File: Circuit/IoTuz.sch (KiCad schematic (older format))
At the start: 29 parts, among them P1 Alligator Connector, P2 BATTERY, P3 USB_5PIN_SHELL, P4 LED_1, P5 LED_2, P6 CONN_01X20, P7 CONN_01X20, Q1 S8050, Q2 S8050, Q3 FDN340P, SW5 RESET, U1 CP2102, U2 ESP32-WROOM

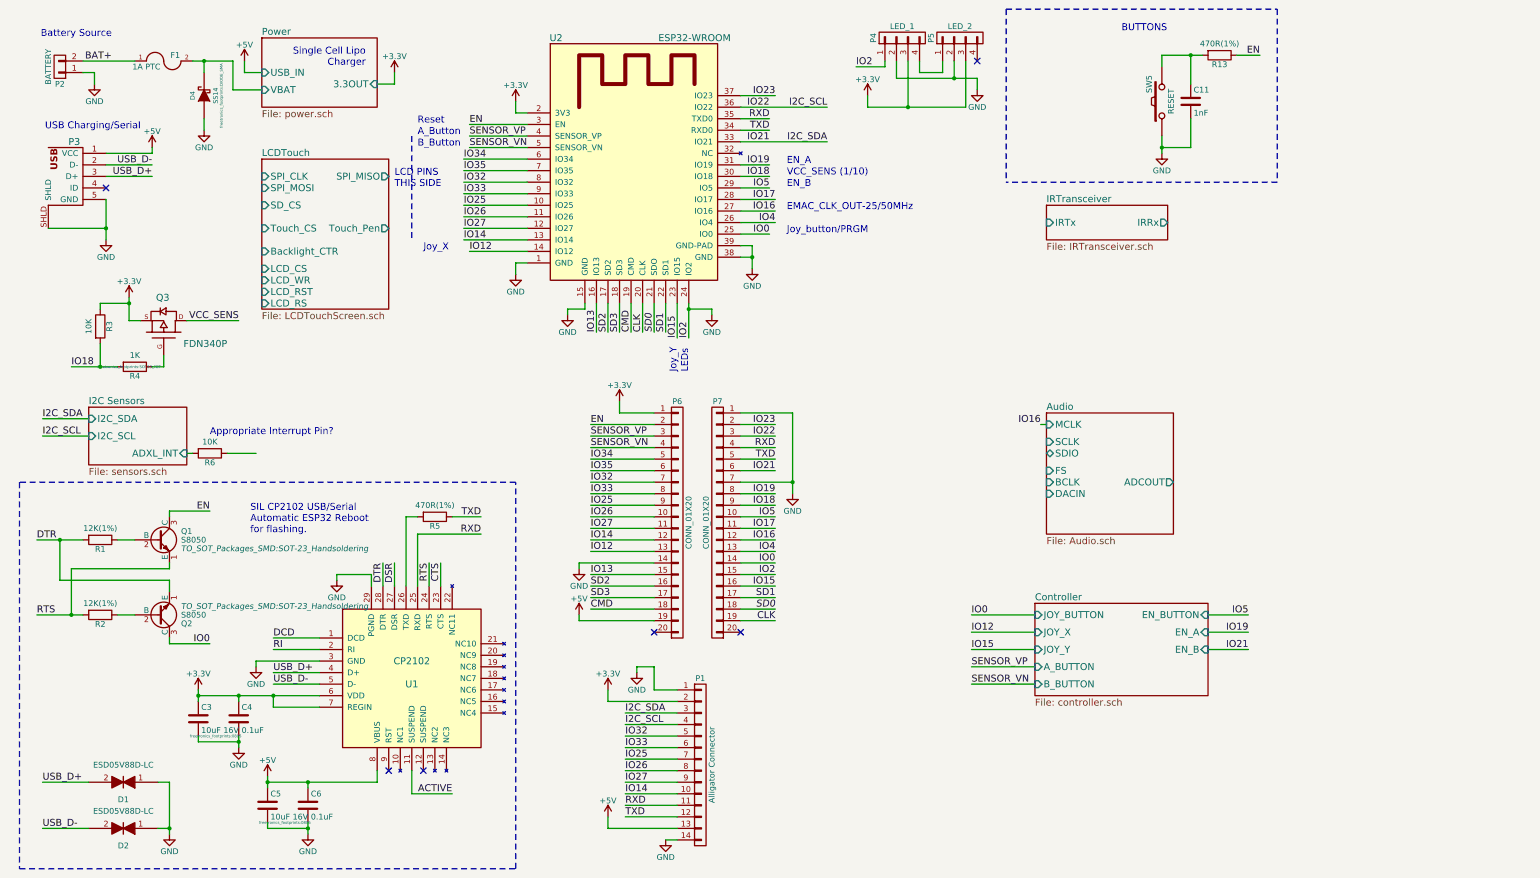
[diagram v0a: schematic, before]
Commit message: Schematic notes.
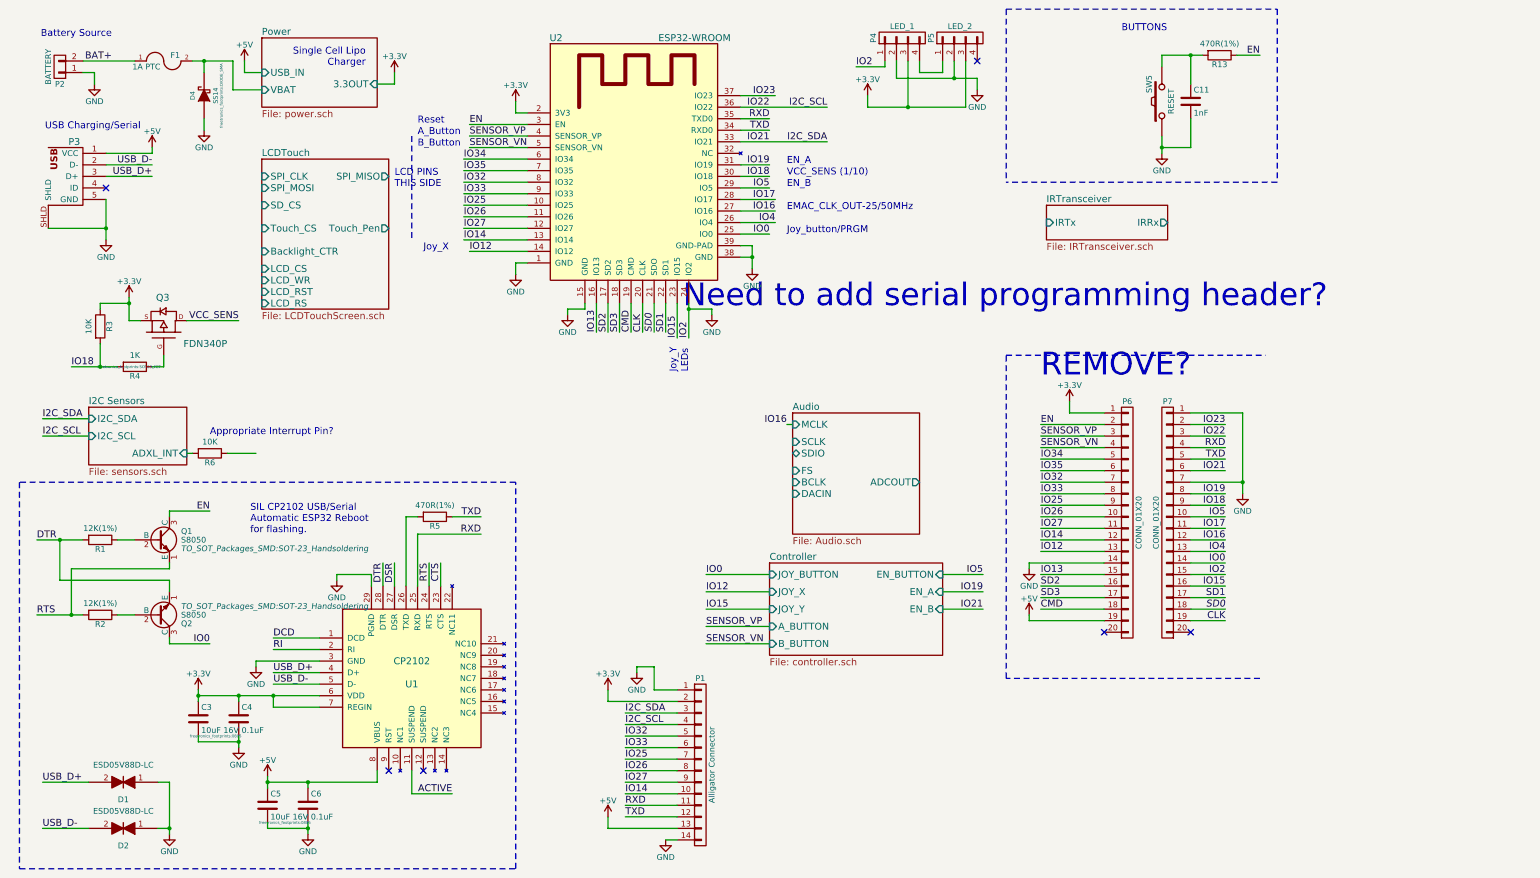
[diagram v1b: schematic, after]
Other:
- note added: "Need to add serial programming header?"
- note added: "REMOVE?"
- moved on the sheet: P6, P7
